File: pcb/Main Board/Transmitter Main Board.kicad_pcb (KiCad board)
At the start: 2 copper layers, 96.5 x 96.5 mm, 37 parts, among them IC1 4960, IC2 4960, IC3 4960, IC4 4960, IC5 4960, IC6 4960, IC7 4960, IC8 4960, J1 Battery, J2 BATTERY MONITOR, J3 Throttle, J4 Steering, J5 VR3, J6 XY JOYSTICK, J7 Neopixel Out, SW1 SW_Push, SW2 SW_Push, SW3 SW_Push, SW4 SW_Push, SW5 SW_Push, SW6 SW_Push, SW7 SW_Push, SW8 SW_Push, U1 Teensy4.1, U2 TLV73312PDBV, U3 NRF24L01_Breakout

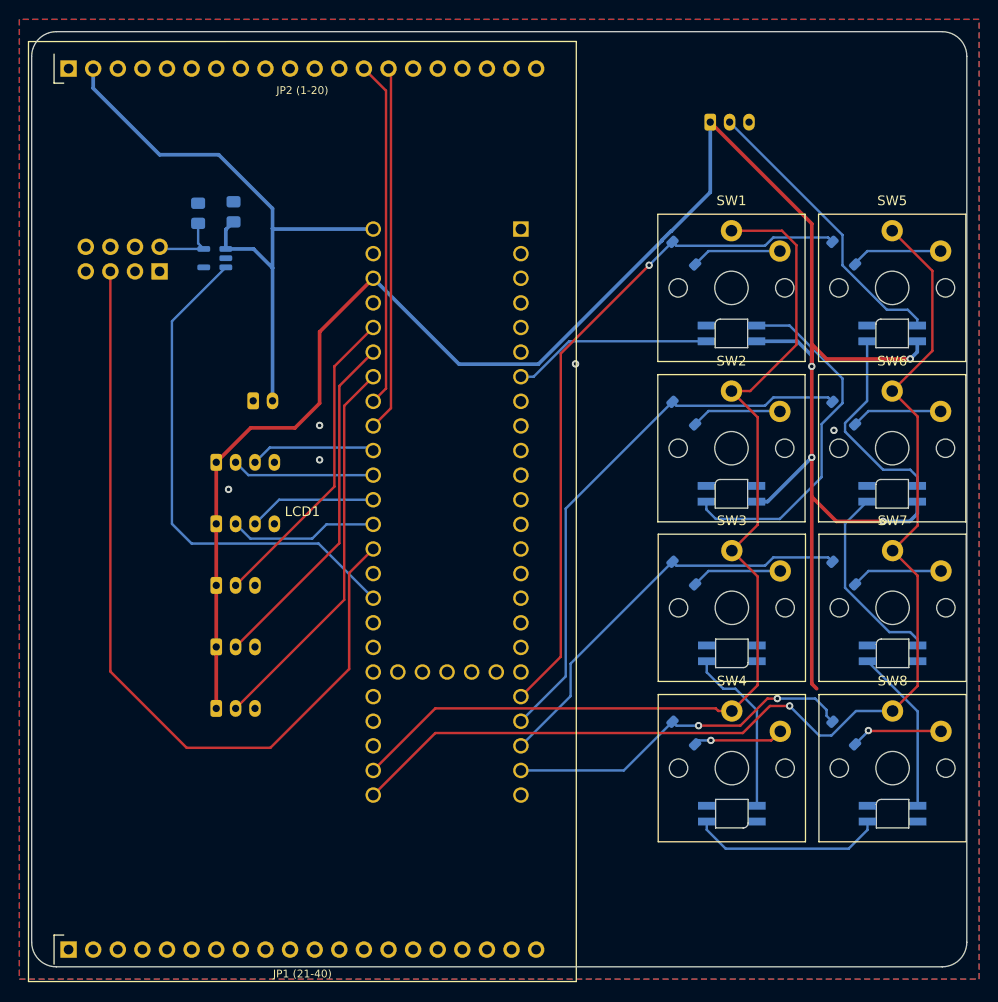
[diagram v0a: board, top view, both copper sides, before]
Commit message: more more more routing
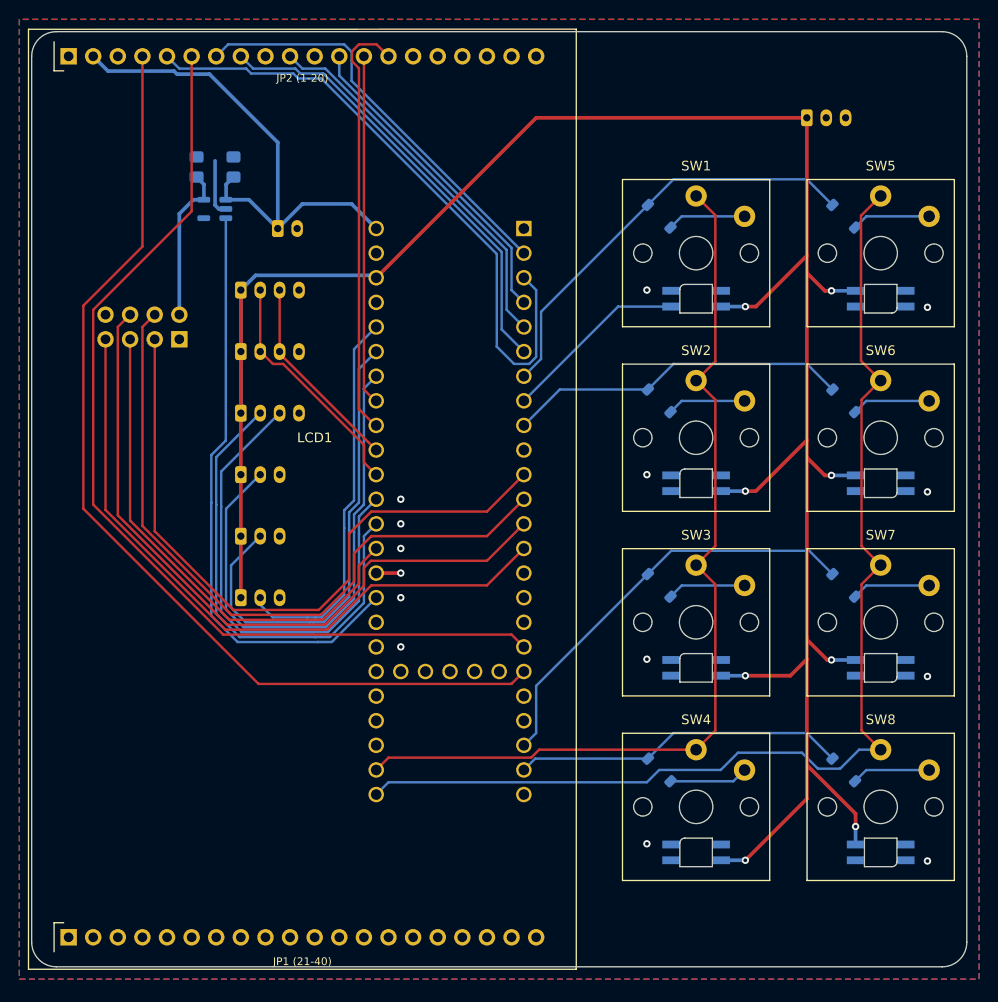
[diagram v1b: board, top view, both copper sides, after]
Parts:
- added J8: Neopixel Out, Connector_JST:JST_PH_B3B-PH-K_1x03_P2.00mm_Vertical, B.Cu at (120.7, 64.8)
- J3: value Throttle -> i2c; footprint Connector_JST:JST_PH_B3B-PH-K_1x03_P2.00mm_Vertical -> Connector_JST:JST_PH_B4B-PH-K_1x04_P2.00mm_Vertical
- J4: value Steering -> Throttle
- J5: value VR3 -> Steering
- J6: value XY JOYSTICK -> VR3; footprint Connector_JST:JST_PH_B4B-PH-K_1x04_P2.00mm_Vertical -> Connector_JST:JST_PH_B3B-PH-K_1x03_P2.00mm_Vertical
- J7: value Neopixel Out -> XY JOYSTICK; footprint Connector_JST:JST_PH_B3B-PH-K_1x03_P2.00mm_Vertical -> Connector_JST:JST_PH_B4B-PH-K_1x04_P2.00mm_Vertical
- moved J7 57.0 mm to (62.2, 95.2)
- moved J3 24.3 mm to (62.2, 88.9)
- moved J1 18.0 mm to (66.0, 76.2)
- moved J2 18.0 mm to (62.2, 82.5)
- moved J5 18.0 mm to (62.2, 108.0)
- moved U3 7.30 mm to (55.9, 87.6)
- moved J6 5.68 mm to (62.2, 101.6)
- moved J4 5.68 mm to (62.2, 114.3)
- moved IC4 5.44 mm to (109.2, 140.6), turned to 180 degrees
- moved SW4 5.44 mm to (109.2, 135.9)
- moved IC1 5.11 mm to (109.2, 83.4)
- moved SW1 5.11 mm to (109.2, 78.7)
- moved U2 5.08 mm to (59.5, 74.2)
- moved C2 4.78 mm to (57.7, 69.8)
- moved C1 4.62 mm to (61.5, 69.8)
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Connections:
- IC5 pad 2: Net-(IC5-DOUT) -> /2x8 Button Matrix/NEO_OUT
- IC5 pad 4: Net-(IC4-DOUT) -> Net-(IC5-DIN)
- IC6 pad 2: Net-(IC6-DOUT) -> Net-(IC5-DIN)
- IC6 pad 4: Net-(IC5-DOUT) -> Net-(IC6-DIN)
- IC7 pad 2: Net-(IC7-DOUT) -> Net-(IC6-DIN)
- IC7 pad 4: Net-(IC6-DOUT) -> Net-(IC7-DIN)
- IC8 pad 2: /2x8 Button Matrix/NEO_OUT -> Net-(IC7-DIN)
- IC8 pad 4: Net-(IC7-DOUT) -> Net-(IC4-DOUT)
- J1 pad 1: GND -> +BATT
- J1 pad 2: +BATT -> GND
- J3 pad 2: /VR1 -> SCL1
- J3 pad 3: GND -> SDA1
- J4 pad 2: /VR2 -> /VR1
- J5 pad 2: /VR3 -> /VR2
- J6 pad 2: /JOY_X -> /VR3
- J6 pad 3: /JOY_Y -> GND
- J7 pad 2: /2x8 Button Matrix/NEO_OUT -> /JOY_X
- J7 pad 3: GND -> /JOY_Y
- U1 pad 20: /ROW_1 -> unconnected-(U1-28_RX7-Pad20)
- U1 pad 21: /ROW_2 -> unconnected-(U1-29_TX7-Pad21)
- U1 pad 4: /TFT_D/C -> /TFT_IRQ
- U1 pad 5: /TFT_IRQ -> /BACKLIGHT
- U1 pad 6: /BACKLIGHT -> /TFT_D/C
- U1 pad 7: /NEOPIXEL -> /ROW_1
- U1 pad 8: unconnected-(U1-6_OUT1D-Pad8) -> /NEOPIXEL
- U1 pad 9: unconnected-(U1-7_RX2_OUT1A-Pad9) -> /ROW_2
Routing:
- net SCK1: track 0.00 -> 102.7 mm
- net MOSI1: track 0.00 -> 101.0 mm
- net MOSI: track 0.00 -> 73.2 mm
- net /RF_CS: track 0.00 -> 72.2 mm
- net /RF_CE: track 0.00 -> 69.8 mm
- net MISO: track 0.00 -> 69.4 mm
- net MISO1: track 0.00 -> 65.8 mm
- net /TFT_D/C: track 0.00 -> 46.5 mm
- net /TFT_CS: track 0.00 -> 43.0 mm
- net /BACKLIGHT: track 0.00 -> 39.3 mm
- net /JOY_Y: track 13.2 -> 50.7 mm
- net Net-(IC1-DOUT): track 37.1 -> 0.00 mm
- net +3.3V: track 215.9 -> 251.6 mm, vias 4 -> 8
- net /JOY_X: track 15.4 -> 49.0 mm
- net SCK: track 86.0 -> 52.5 mm
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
